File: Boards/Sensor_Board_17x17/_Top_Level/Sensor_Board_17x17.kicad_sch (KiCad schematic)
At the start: 80 parts, among them J1 OQ0212500000G, J10 OQ0212500000G, J11 OQ0212500000G, J12 OQ0212500000G, J13 OQ0212500000G, J14 OQ0212500000G, J15 OQ0212500000G, J16 OQ0212500000G, J2 OQ0212500000G, J3 OQ0212500000G, J4 OQ0212500000G, J5 OQ0212500000G, J6 OQ0212500000G, J7 OQ0212500000G, J8 OQ0212500000G, J9 OQ0212500000G

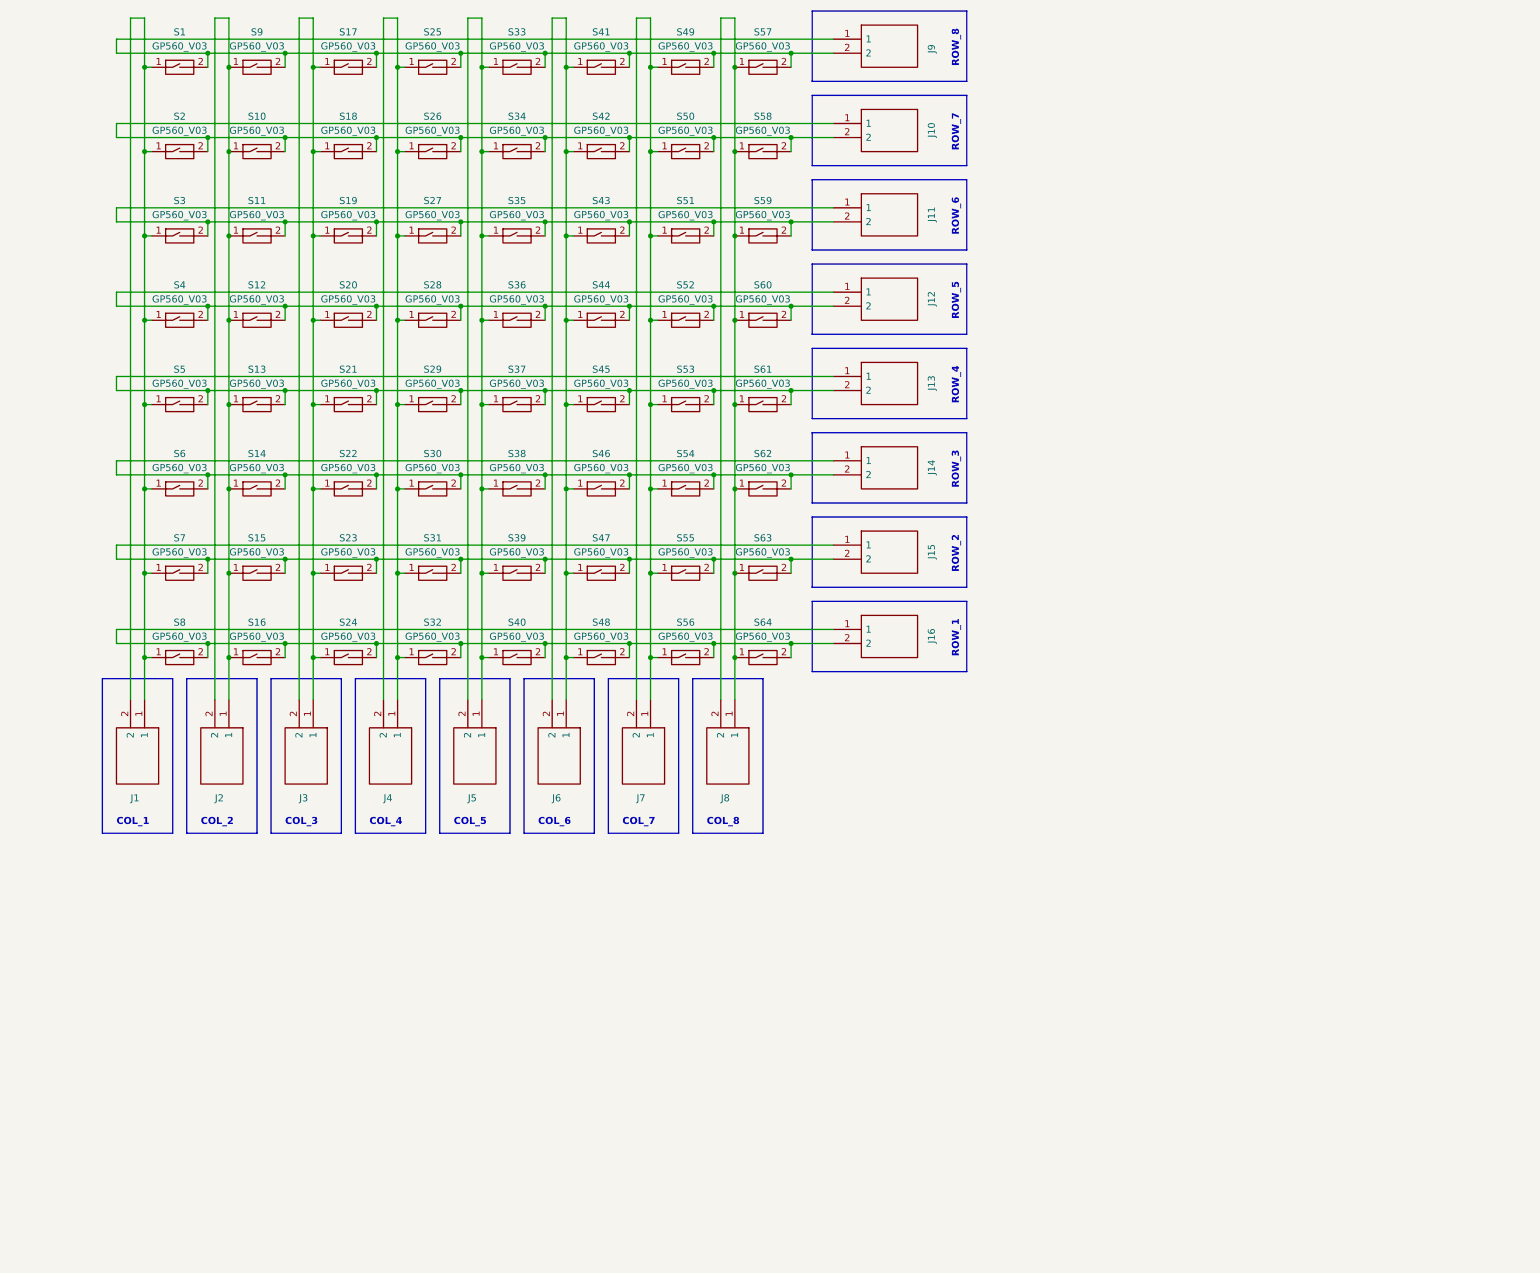
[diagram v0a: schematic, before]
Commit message: Changes for sensor network
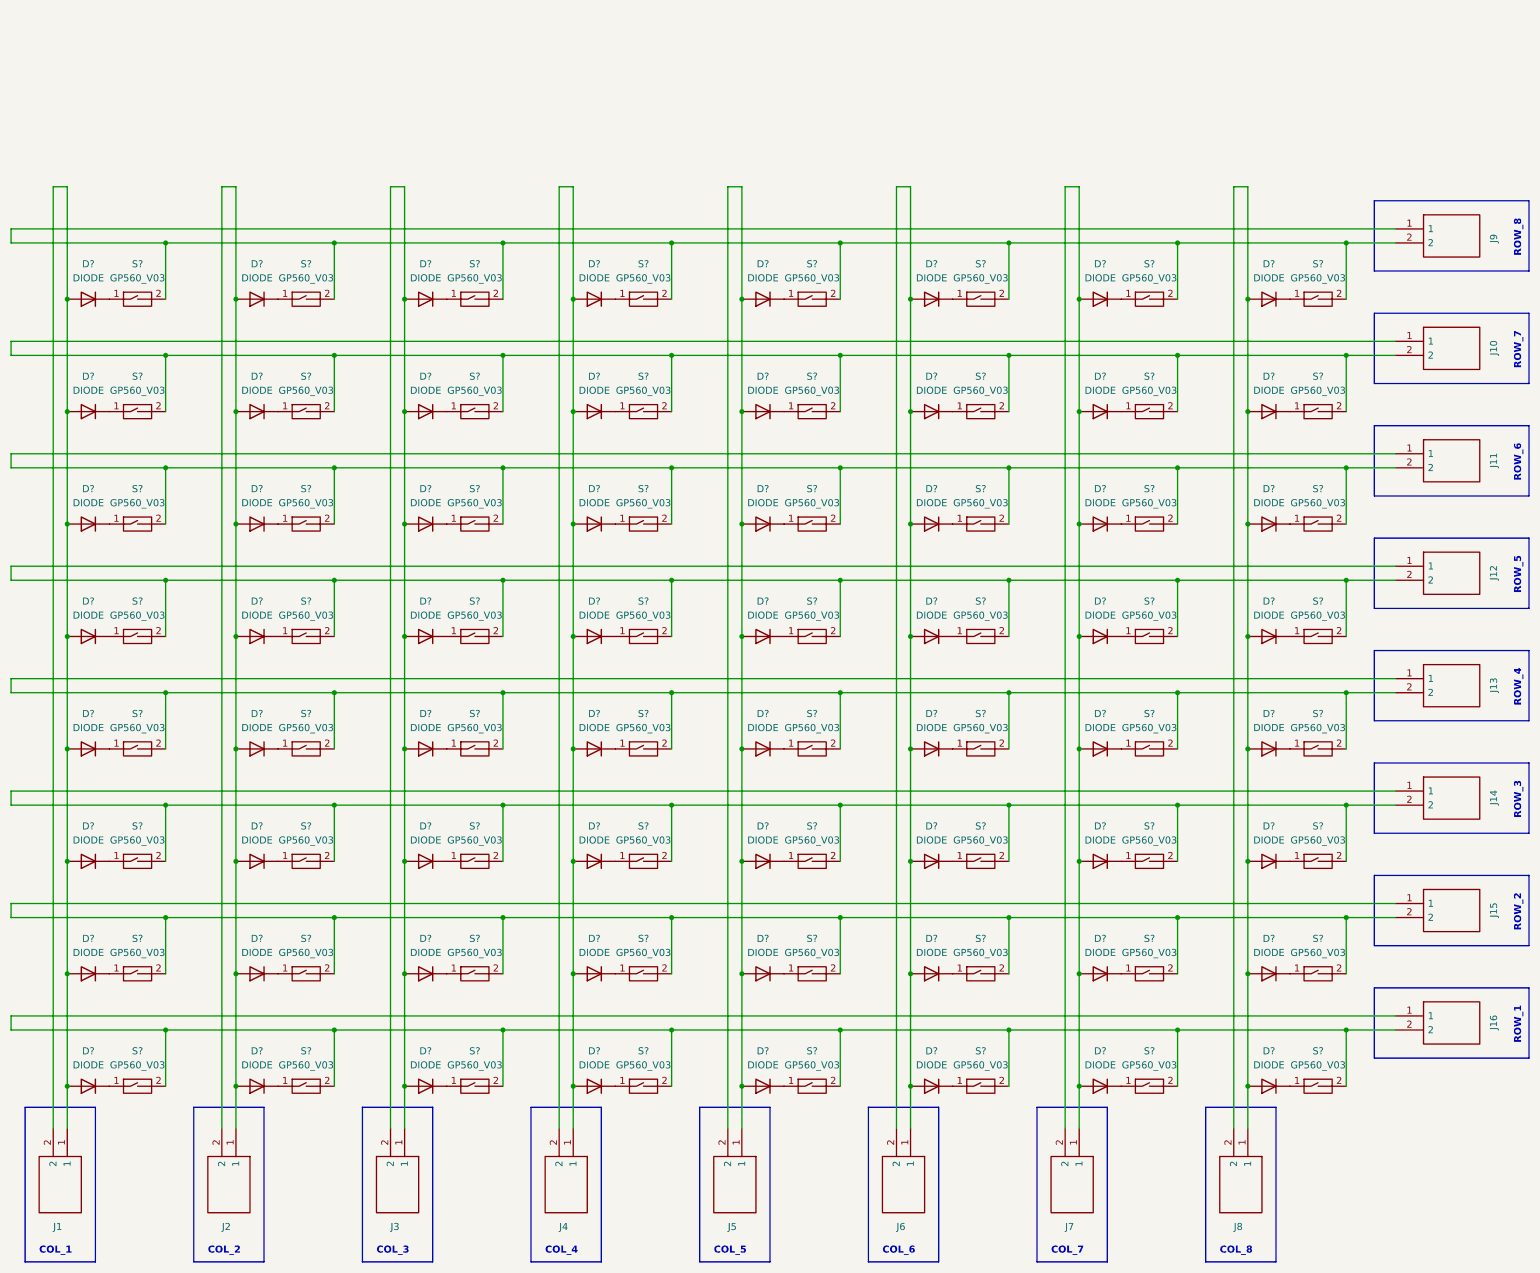
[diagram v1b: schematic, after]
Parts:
- removed S1, S10, S11, S12, S13, S14, S15, S16, S17, S18, S19, S2, S20, S21, S22, S23, S24, S25, S26, S27, S28, S29, S3, S30, S31, S32, S33, S34, S35, S36, S37, S38, S39, S4, S40, S41, S42, S43, S44, S45, S46, S47, S48, S49, S5, S50, S51, S52, S53, S54, S55, S56, S57, S58, S59, S6, S60, S61, S62, S63, S64, S7, S8, S9: GP560_V03, GP560_V03:GP560_V03, symbol GP560_V03:GP560_V03
- added D? (x64): DIODE, symbol Simulation_SPICE:DIODE
- added S? (x64): GP560_V03, GP560_V03:GP560_V03, symbol GP560_V03:GP560_V03
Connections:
- net at J6.1, J6.2: now also D?.1 (A), D?.1 (A), D?.1 (A), D?.1 (A), D?.1 (A), D?.1 (A), D?.1 (A), D?.1 (A)
- net at J9.1, J9.2: now also S?.2, S?.2, S?.2, S?.2, S?.2, S?.2, S?.2, S?.2
- net at J1.1, J1.2: now also D?.1 (A), D?.1 (A), D?.1 (A), D?.1 (A), D?.1 (A), D?.1 (A), D?.1 (A), D?.1 (A)
- net at J16.1, J16.2: now also S?.2, S?.2, S?.2, S?.2, S?.2, S?.2, S?.2, S?.2
- net at J2.1, J2.2: now also D?.1 (A), D?.1 (A), D?.1 (A), D?.1 (A), D?.1 (A), D?.1 (A), D?.1 (A), D?.1 (A)
- net at J13.1, J13.2: now also S?.2, S?.2, S?.2, S?.2, S?.2, S?.2, S?.2, S?.2
- net at J12.1, J12.2: now also S?.2, S?.2, S?.2, S?.2, S?.2, S?.2, S?.2, S?.2
- net at J8.1, J8.2: now also D?.1 (A), D?.1 (A), D?.1 (A), D?.1 (A), D?.1 (A), D?.1 (A), D?.1 (A), D?.1 (A)
- net at J11.1, J11.2: now also S?.2, S?.2, S?.2, S?.2, S?.2, S?.2, S?.2, S?.2
- net at J7.1, J7.2: now also D?.1 (A), D?.1 (A), D?.1 (A), D?.1 (A), D?.1 (A), D?.1 (A), D?.1 (A), D?.1 (A)
- net at J15.1, J15.2: now also S?.2, S?.2, S?.2, S?.2, S?.2, S?.2, S?.2, S?.2
- net at J10.1, J10.2: now also S?.2, S?.2, S?.2, S?.2, S?.2, S?.2, S?.2, S?.2
- net at J5.1, J5.2: now also D?.1 (A), D?.1 (A), D?.1 (A), D?.1 (A), D?.1 (A), D?.1 (A), D?.1 (A), D?.1 (A)
- net at J3.1, J3.2: now also D?.1 (A), D?.1 (A), D?.1 (A), D?.1 (A), D?.1 (A), D?.1 (A), D?.1 (A), D?.1 (A)
- net at J14.1, J14.2: now also S?.2, S?.2, S?.2, S?.2, S?.2, S?.2, S?.2, S?.2
- net at J4.1, J4.2: now also D?.1 (A), D?.1 (A), D?.1 (A), D?.1 (A), D?.1 (A), D?.1 (A), D?.1 (A), D?.1 (A)
- new net: D?.2 (K), S?.1 (x64)
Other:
- moved on the sheet: J1, J10, J11, J12, J13, J14, J15, J16, J2, J3, J4, J5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
